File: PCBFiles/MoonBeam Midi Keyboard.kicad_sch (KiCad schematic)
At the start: 98 parts, among them J1 LED Matrix, J2 AudioJack4_SwitchTR1, J3 Conn_01x01_Pin, J4 Conn_01x01_Pin, J5 Conn_01x01_Pin, J6 Conn_01x01_Pin, J7 Conn_01x01_Pin, SW1 SW_Omron_B3FS, SW10 SW_Omron_B3FS, SW11 SW_Omron_B3FS, SW13 SW_Omron_B3FS, SW14 SW_Omron_B3FS, SW15 SW_Omron_B3FS, SW16 SW_Omron_B3FS, SW17 SW_Omron_B3FS, SW18 SW_Omron_B3FS, SW19 SW_Omron_B3FS, SW2 SW_Omron_B3FS, SW20 SW_Omron_B3FS, SW21 SW_Omron_B3FS, SW22 SW_Omron_B3FS, SW25 SW_Omron_B3FS, SW27 SW_Omron_B3FS, SW29 SW_Omron_B3FS, SW3 SW_Omron_B3FS, SW31 SW_Omron_B3FS, SW33 SW_Omron_B3FS, SW37 RotaryEncoder_Switch_MP, SW38 RotaryEncoder_Switch_MP, SW4 SW_Omron_B3FS, SW5 SW_Omron_B3FS, SW6 SW_SPDT, SW7 SW_Omron_B3FS, SW8 SW_Omron_B3FS, SW9 SW_Omron_B3FS, U2 PCM5100, U3 LM4810, U4 LM4861

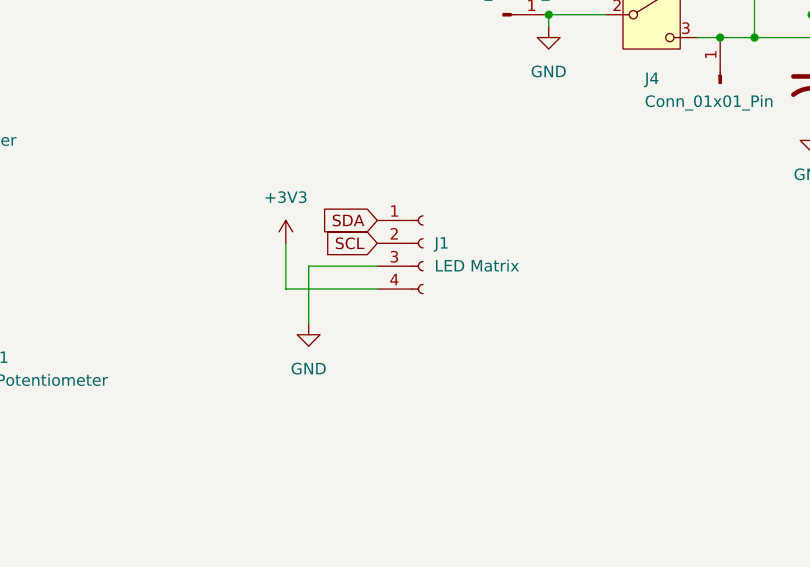
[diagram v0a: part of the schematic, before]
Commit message: added updated PCB files
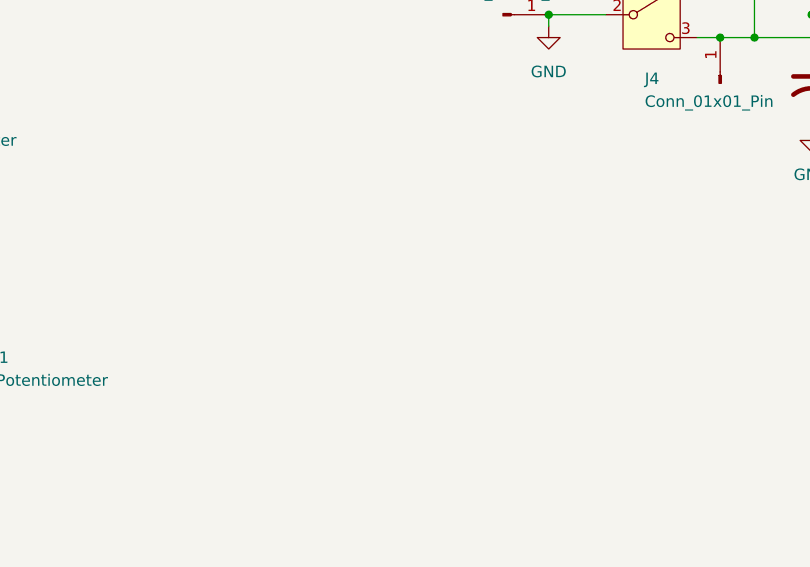
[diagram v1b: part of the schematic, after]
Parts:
- removed J1: LED Matrix, Connector_PinHeader_2.54mm:PinHeader_1x04_P2.54mm_Vertical, symbol Connector:Conn_01x04_Socket
- R1, R10, R11, R2, R3, R4, R5, R6, R7, R8, R9: footprint Resistor_THT:R_Axial_DIN0207_L6.3mm_D2.5mm_P7.62mm_Horizontal -> Resistor_THT:R_Axial_DIN0207_L6.3mm_D2.5mm_P10.16mm_Horizontal
